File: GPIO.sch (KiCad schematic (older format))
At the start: 21 parts, among them J1 MICROUSB, P1 CONN_12, Q2 FDD8870, SW1 SW_PUSH_SMALL, SW2 SW_PUSH_SMALL, SW3 SW_PUSH_SMALL

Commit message: Main sheet integration progress
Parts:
- removed J1: MICROUSB, symbol MICROUSB
- removed Q2: FDD8870, symbol MOSFET_N
- removed R2: 10K, symbol R
- removed U?: MC78M05, ~, symbol MC78M05
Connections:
- net labels added: Battery+, Battery-, Gate, Vout
- net labels removed: +Vcc, Battery1+, Battery1-, Battery2+, Battery2-, Switch-, Vbus
- wire segments 88 -> 53
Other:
- moved on the sheet: R?

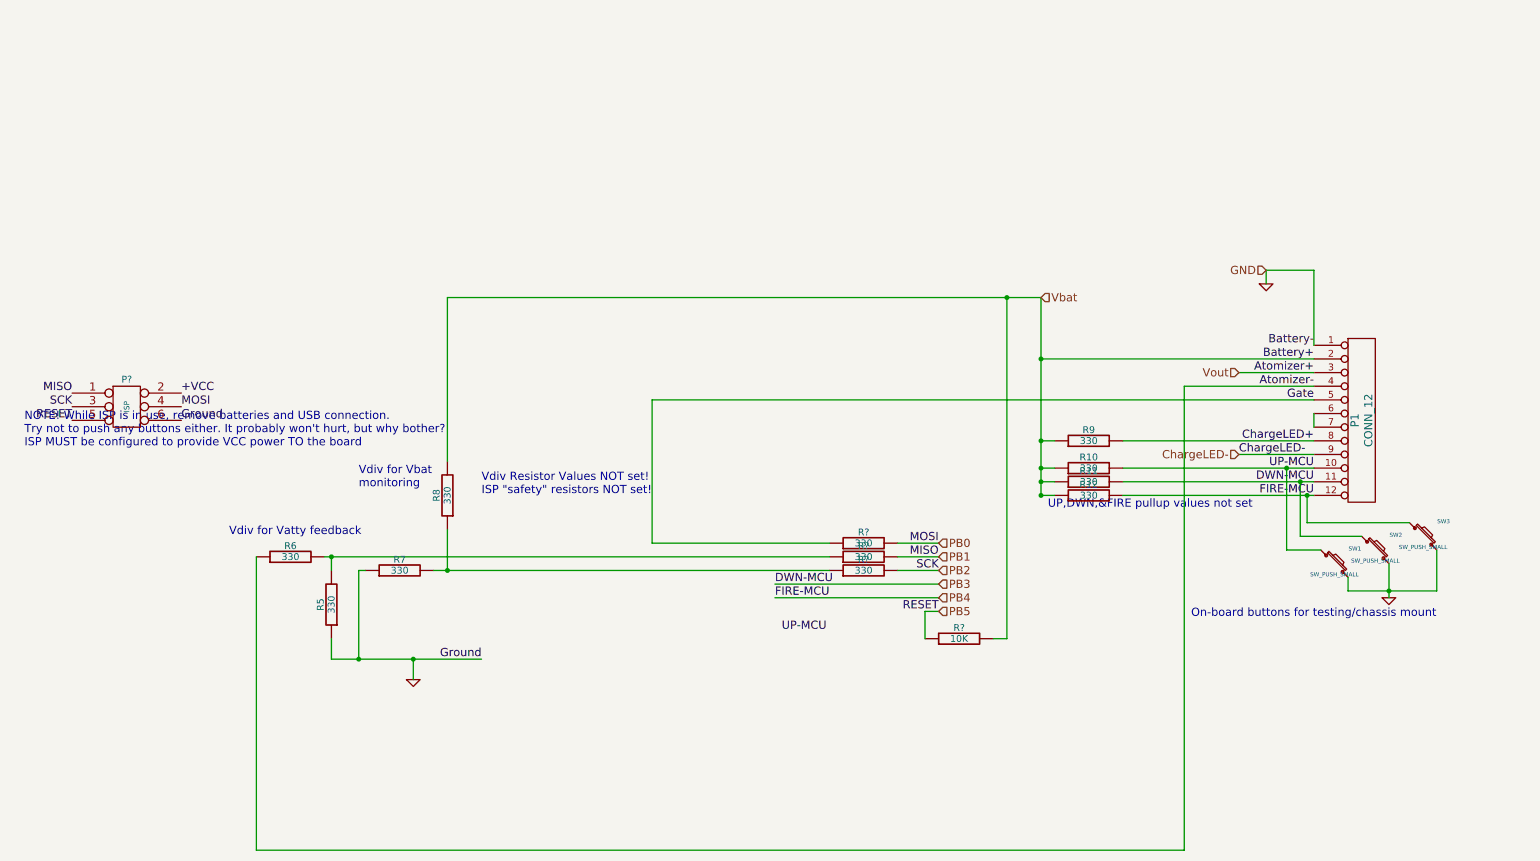
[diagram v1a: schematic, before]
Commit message: adsf
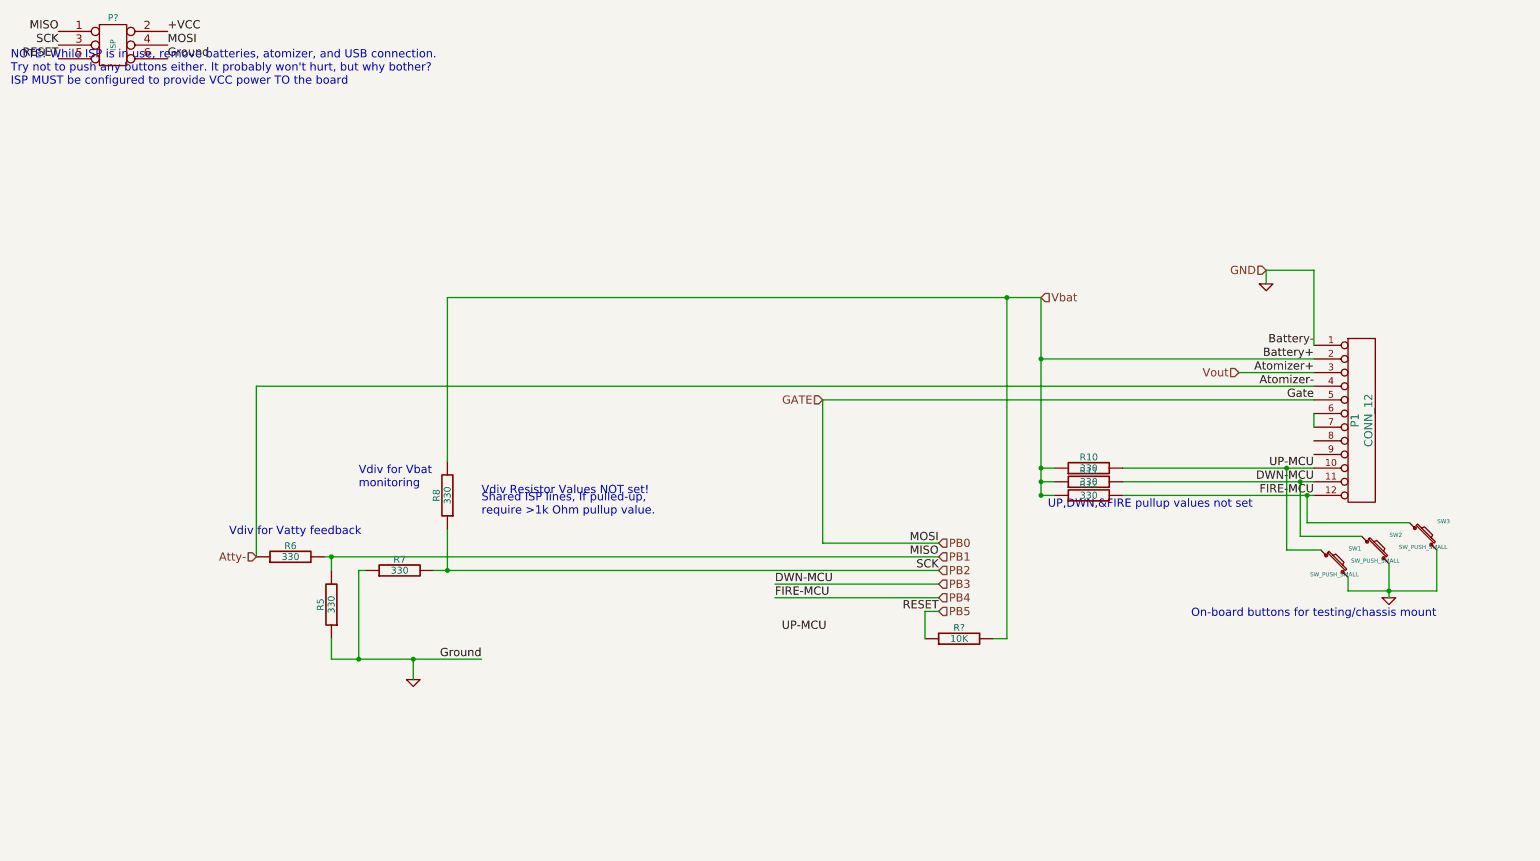
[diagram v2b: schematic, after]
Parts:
- removed R9, R? (x3): 330, symbol R
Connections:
- net PB0 is gone; now on net GATE: P?.4
- net PB1: now also R5.2, R6.2
- net PB2: now also R7.2, R8.1
- net Atomizer- renamed Atty-
- net ChargeLED+: no longer names the net of P1.8 (P8)
- net ChargeLED-: no longer names the net of P1.9 (P9)
- net Gate renamed GATE
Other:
- note added: "NOTE! While ISP is in use, remove batteries, atomizer, and USB connection.\nTry not to push any buttons either. It probably won't hurt, but why bother?\nISP MUST be configured to provide VCC power TO the board"
- note added: "Shared ISP lines, If pulled-up, \nrequire >1k Ohm pullup value."
- note added: "Vdiv Resistor Values NOT set!"
- note removed: "NOTE! While ISP is in use, remove batteries and USB connection.\nTry not to push any buttons either. It probably won't hurt, but why bother?\nISP MUST be configured to provide VCC power TO the board"
- note removed: "Vdiv Resistor Values NOT set!\nISP "safety" resistors NOT set!"
- moved on the sheet: P?
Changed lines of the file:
@@
-EESchema Schematic File Version 2  date Thu 04 Apr 2013 10:55:40 AM CDT
+EESchema Schematic File Version 2  date Fri 05 Apr 2013 11:43:57 PM CDT
 LIBS:power
 LIBS:device
@@
 Sheet 4 4
 Title ""
-Date "4 apr 2013"
+Date "5 apr 2013"
 Rev ""
 Comp ""
@@
 	1    0    0    -1
 $EndComp
-$Comp
-L R R9
-U 1 1 5155E6A2
-P 8400 3700
-F 0 "R9" V 8480 3700 50  0000 C CNN
-F 1 "330" V 8400 3700 50  0000 C CNN
-F 2 "" H 8400 3700 60  0001 C CNN
-F 3 "" H 8400 3700 60  0001 C CNN
-	1    8400 3700
-	0    -1   -1   0
-$EndComp
-Text Label 10050 3700 2    60   ~ 0
-ChargeLED+
-Text Label 9500 3800 0    60   ~ 0
-ChargeLED-
 Text Label 10050 3300 2    60   ~ 0
 Atomizer-
@@
 L CONN_3X2 P?
 U 1 1 515A2371
-P 1350 3500
-F 0 "P?" H 1350 3750 50  0000 C CNN
-F 1 "ISP" V 1350 3550 40  0000 C CNN
-F 2 "" H 1350 3500 60  0000 C CNN
-F 3 "" H 1350 3500 60  0000 C CNN
-	1    1350 3500
-	1    0    0    -1
-$EndComp
-Text Label 950  3350 2    60   ~ 0
+P 1250 850
+F 0 "P?" H 1250 1100 50  0000 C CNN
+F 1 "ISP" V 1250 900 40  0000 C CNN
+F 2 "" H 1250 850 60  0000 C CNN
+F 3 "" H 1250 850 60  0000 C CNN
+	1    1250 850
+	1    0    0    -1
+$EndComp
+Text Label 850  700  2    60   ~ 0
 MISO
-Text Label 950  3450 2    60   ~ 0
+Text Label 850  800  2    60   ~ 0
 SCK
-Text Label 950  3550 2    60   ~ 0
+Text Label 850  900  2    60   ~ 0
 RESET
-Text Label 1750 3350 0    60   ~ 0
+Text Label 1650 700  0    60   ~ 0
 +VCC
-Text Label 1750 3450 0    60   ~ 0
+Text Label 1650 800  0    60   ~ 0
 MOSI
-Text Label 1750 3550 0    60   ~ 0
+Text Label 1650 900  0    60   ~ 0
 Ground
 Text Label 3950 5300 2    60   ~ 0
@@
 Text Label 7300 4950 2    60   ~ 0
 RESET
-Text Notes 600  3750 0    60   ~ 0
-NOTE! While ISP is in use, remove batteries and USB connection.\nTry not to push any buttons either. It probably won't hurt, but why bother?\nISP MUST be configured to provide VCC power TO the board
-$Comp
-L R R?
-U 1 1 515C4802
-P 6750 4450
-F 0 "R?" V 6830 4450 50  0000 C CNN
-F 1 "330" V 6750 4450 50  0000 C CNN
-F 2 "" H 6750 4450 60  0001 C CNN
-F 3 "" H 6750 4450 60  0001 C CNN
-	1    6750 4450
-	0    -1   -1   0
-$EndComp
-$Comp
-L R R?
-U 1 1 515C4811
-P 6750 4550
-F 0 "R?" V 6830 4550 50  0000 C CNN
-F 1 "330" V 6750 4550 50  0000 C CNN
-F 2 "" H 6750 4550 60  0001 C CNN
-F 3 "" H 6750 4550 60  0001 C CNN
-	1    6750 4550
-	0    -1   -1   0
-$EndComp
-$Comp
-L R R?
-U 1 1 515C4820
-P 6750 4650
-F 0 "R?" V 6830 4650 50  0000 C CNN
-F 1 "330" V 6750 4650 50  0000 C CNN
-F 2 "" H 6750 4650 60  0001 C CNN
-F 3 "" H 6750 4650 60  0001 C CNN
-	1    6750 4650
-	0    -1   -1   0
-$EndComp
+Text Notes 500  1100 0    60   ~ 0
+NOTE! While ISP is in use, remove batteries, atomizer, and USB connection.\nTry not to push any buttons either. It probably won't hurt, but why bother?\nISP MUST be configured to provide VCC power TO the board
 Text Notes 3950 4100 0    60   ~ 0
-Vdiv Resistor Values NOT set!\nISP "safety" resistors NOT set!
+Vdiv Resistor Values NOT set!
 Text HLabel 8050 2650 2    60   Input ~ 0
 Vbat
@@
 	0    -1   -1   0
 $EndComp
-Text HLabel 9500 3800 0    60   Input ~ 0
-ChargeLED-
 Text Label 10050 3400 2    60   ~ 0
 Gate
@@
 	3450 5300 3450 5450
 Wire Wire Line
-	2850 5300 3950 5300
+	2850 5300 3050 5300
+Wire Wire Line
+	3050 5300 3450 5300
+Wire Wire Line
+	3450 5300 3950 5300
 Connection ~ 3450 5300
 Wire Wire Line
-	2300 6700 9100 6700
-Wire Wire Line
-	9100 6700 9100 3300
-Wire Wire Line
 	3700 4350 3700 4650
 Wire Wire Line
-	2300 4550 2300 6700
-Wire Wire Line
-	2800 4550 6500 4550
+	2800 4550 2850 4550
+Wire Wire Line
+	2850 4550 7300 4550
 Wire Wire Line
 	2850 5150 2850 5300
 Wire Wire Line
-	3600 4650 6500 4650
+	3600 4650 3700 4650
+Wire Wire Line
+	3700 4650 7300 4650
 Connection ~ 3700 4650
 Wire Wire Line
-	8650 4100 10050 4100
+	8650 4100 10000 4100
+Wire Wire Line
+	10000 4100 10050 4100
 Wire Wire Line
 	3100 4650 3050 4650
@@
 Connection ~ 8050 4100
 Wire Wire Line
-	8650 4000 10050 4000
-Wire Wire Line
-	8650 3900 10050 3900
+	8650 4000 9950 4000
+Wire Wire Line
+	9950 4000 10050 4000
+Wire Wire Line
+	8650 3900 9850 3900
+Wire Wire Line
+	9850 3900 10050 3900
 Wire Wire Line
 	7300 4750 6100 4750
@@
 	10750 4300 10000 4300
 Wire Wire Line
-	10600 4600 10600 4850
+	10600 4600 10600 4800
+Wire Wire Line
+	10600 4800 10600 4850
 Wire Wire Line
 	10300 4700 10300 4800
 Wire Wire Line
-	10300 4800 10950 4800
+	10300 4800 10600 4800
+Wire Wire Line
+	10600 4800 10950 4800
 Connection ~ 10600 4800
 Wire Wire Line
 	10950 4800 10950 4500
-Wire Wire Line
-	8050 3700 8150 3700
-Connection ~ 8050 3700
-Wire Wire Line
-	8650 3700 10050 3700
-Wire Wire Line
-	10050 3800 9500 3800
 Wire Wire Line
 	2850 4550 2850 4650
@@
 	3700 2650 3700 3850
 Wire Wire Line
-	3700 2650 8050 2650
-Wire Wire Line
-	8050 2650 8050 4100
-Wire Wire Line
-	7300 4450 7000 4450
-Wire Wire Line
-	7000 4550 7300 4550
-Wire Wire Line
-	7300 4650 7000 4650
-Wire Wire Line
-	5200 4450 6500 4450
+	3700 2650 7800 2650
+Wire Wire Line
+	7800 2650 8050 2650
+Wire Wire Line
+	8050 2650 8050 3100
+Wire Wire Line
+	8050 3100 8050 3900
+Wire Wire Line
+	8050 3900 8050 4000
+Wire Wire Line
+	8050 4000 8050 4100
+Wire Wire Line
+	6450 4450 7300 4450
 Wire Wire Line
 	7700 5150 7800 5150
 Wire Wire Line
 	7800 5150 7800 2650
-Wire Wire Line
-	9100 3300 10050 3300
 Connection ~ 7800 2650
 Wire Wire Line
-	10050 3400 5200 3400
-Wire Wire Line
-	5200 3400 5200 4450
+	10050 3400 6450 3400
+Wire Wire Line
+	6450 3400 6450 4450
 Wire Wire Line
 	7200 5150 7200 4950
@@
 Text HLabel 9700 2450 0    60   Input ~ 0
 GND
+Text Notes 3950 4250 0    60   ~ 0
+Shared ISP lines, If pulled-up, \nrequire >1k Ohm pullup value.
+Wire Wire Line
+	10050 3300 2300 3300
+Wire Wire Line
+	2300 3300 2300 4550
+Text HLabel 6450 3400 0    60   Input ~ 0
+GATE
+Text HLabel 2300 4550 0    60   Input ~ 0
+Atty-
 $EndSCHEMATC
